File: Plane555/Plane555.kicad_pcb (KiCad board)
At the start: 2 copper layers, 106.6 x 90.2 mm, 32 parts, among them SW1 SW_SPDT

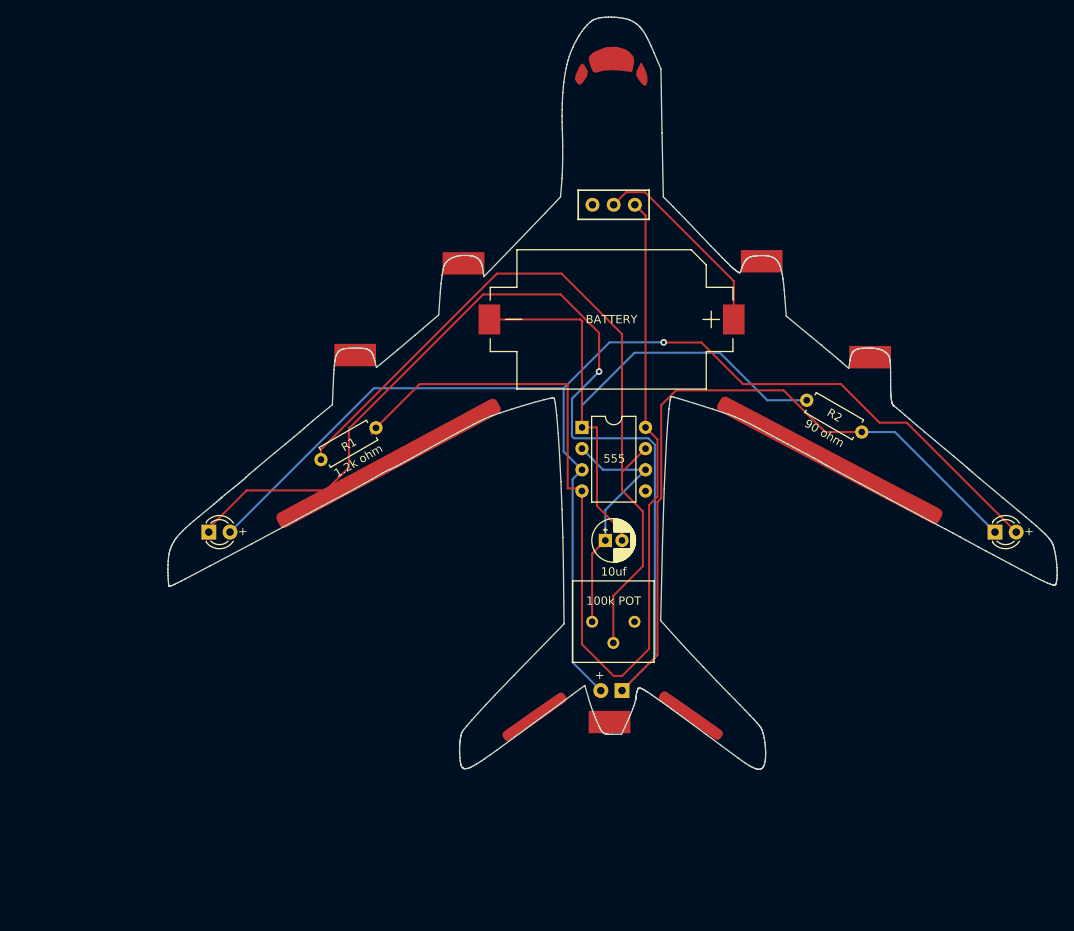
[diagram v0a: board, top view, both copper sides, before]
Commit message: feat: init new files
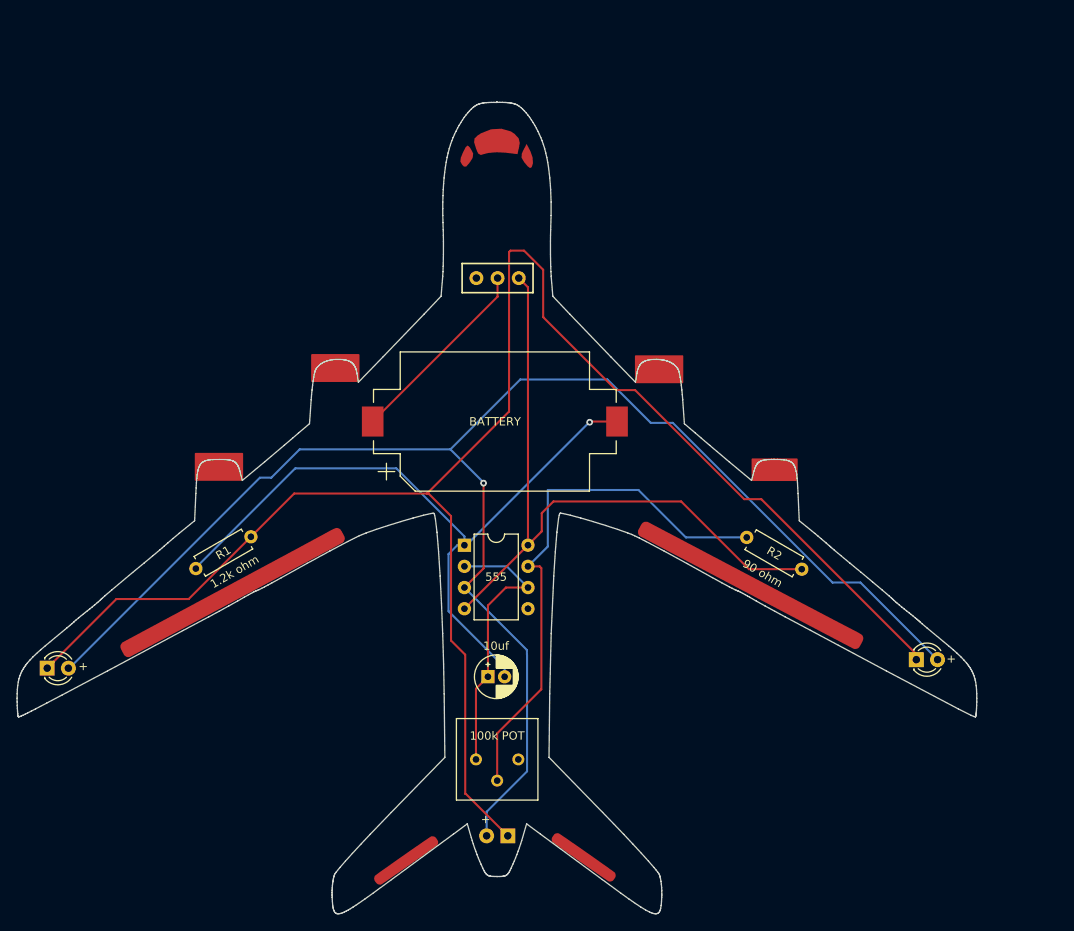
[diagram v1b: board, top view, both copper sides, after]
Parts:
- removed the G*** at (121.5, 67.0) (x2)
- removed the G*** at (170.2, 78.2) (x2)
- removed the G*** at (149.2, 123.2) (x2)
- removed the G*** at (139.2, 43.2) (x2)
- removed the G*** at (132.0, 121.6) (x2)
- removed the G*** at (108.5, 78.0) (x2)
- removed the G*** at (165.2, 90.2) (x2)
- removed the G*** at (139.0, 122.0) (x2)
- removed the G*** at (112.1, 90.9) (x2)
- removed the G*** at (139.5, 84.5)
- removed the G*** at (157.2, 66.8) (x2)
- removed RV1: 100k POT, Potentiometer_THT:Potentiometer_Bourns_3386P_Vertical
- added 100k POT: POT, Potentiometer_THT:Potentiometer_Bourns_3386P_Vertical, F.Cu at (123.0, 126.5)
- added G*** (x2): LOGO, LOGO, F.Cu at (136.4, 140.2)
- added G*** (x2): LOGO, LOGO, F.Cu at (155.8, 105.2)
- added G***: LOGO, LOGO, B.Cu at (125.7, 97.5)
- added G*** (x2): LOGO, LOGO, F.Cu at (116.6, 138.9)
- added G*** (x2): LOGO, LOGO, F.Cu at (125.5, 53.1)
- added G*** (x2): LOGO, LOGO, F.Cu at (93.4, 106.4)
- C1: value 10uf -> 10uf
- D1: footprint LED_THT:LED_D3.0mm -> LED_THT:LED_D3.0mm_Horizontal_O1.27mm_Z2.0mm; moved to B.Cu
- D3: footprint LED_THT:LED_D3.0mm_Horizontal_O1.27mm_Z2.0mm -> LED_THT:LED_D3.0mm; moved to F.Cu
- SW1: footprint SW SS12D:Schiebeschalter SS-12D00.kicad_mod -> Button_Switch_THT:Schiebeschalter_SS-12D00
- moved D2 114.8 mm to (71.6, 115.6)
- moved D1 51.1 mm to (126.8, 135.7), turned to 180 degrees
- moved D3 35.5 mm to (175.8, 114.5), turned to 0 degrees
- moved C1 21.6 mm to (124.4, 116.6)
- moved 555 19.9 mm to (121.6, 100.8)
- moved R1 19.9 mm to (89.4, 103.6)
- moved ? 19.3 mm to (146.8, 91.6), turned to 0 degrees
- moved BATTERY 18.6 mm to (125.3, 86.0), turned to 0 degrees
- moved R2 18.0 mm to (155.5, 99.9)
- moved SW1 16.5 mm to (125.6, 68.8)
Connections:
- R1 pad 1: Net-(U1-DIS) -> GNDREF
- R1 pad 2: +3V0 -> Net-(D1-K)
- R2 pad 1: GNDREF -> Net-(U1-DIS)
- R2 pad 2: Net-(D1-K) -> +3V0
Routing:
- net +3V0: track 124.6 -> 82.9 mm
- net Net-(D1-A): track 152.1 -> 186.6 mm
- net Net-(U1-DIS): track 92.6 -> 65.7 mm
- net GNDREF: track 75.1 -> 86.0 mm, vias 0 -> 1
- net Net-(U1-THR): track 29.5 -> 33.4 mm
- net Net-(D1-K): track 202.9 -> 205.4 mm, vias 1 -> 0
- net Net-(BT1-+): track 24.0 -> 23.4 mm
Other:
- board size 106.6 x 90.2 mm -> 115.1 x 97.3 mm
